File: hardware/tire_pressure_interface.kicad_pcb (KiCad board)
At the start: 2 copper layers, 98 x 40.1 mm, 82 parts, among them IC1 TPS54202HDDCR, J3 FTSH-107-01-L-D-K, J4 Conn_02x02_Counter_Clockwise, J5 Micro_SD_Card_Det1, Q1 SI2347DS-T1-GE3, T1 TP_+3V3, T10 TP_+5V, T11 TP_+5V, T3 TP_VCC, T8 TP_VCC, T9 TP_+3V3, U1 STM32G0C1KCTxN, U2 LM1117-3.3, U3 XIAO-ESP32-S3-DIP, U7 ADM3057ExRW

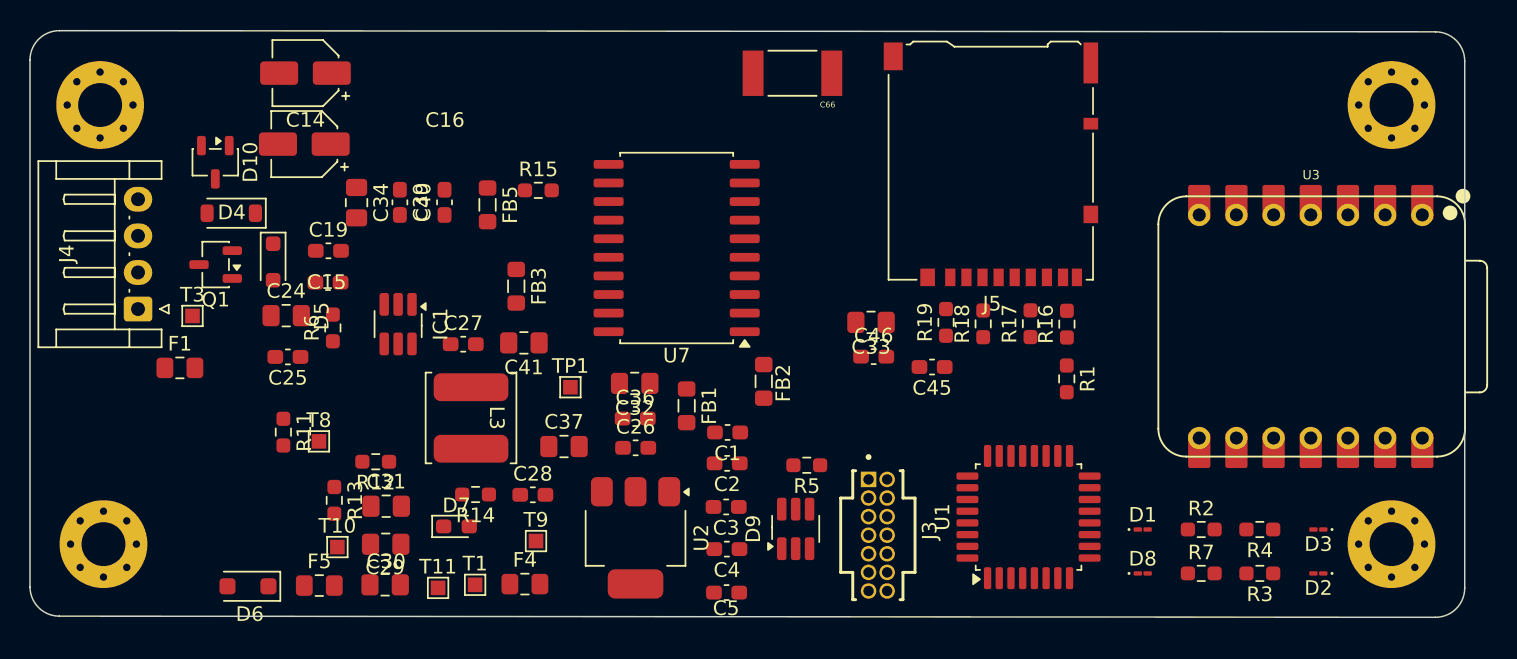
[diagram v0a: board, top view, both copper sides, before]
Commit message: pcb routing
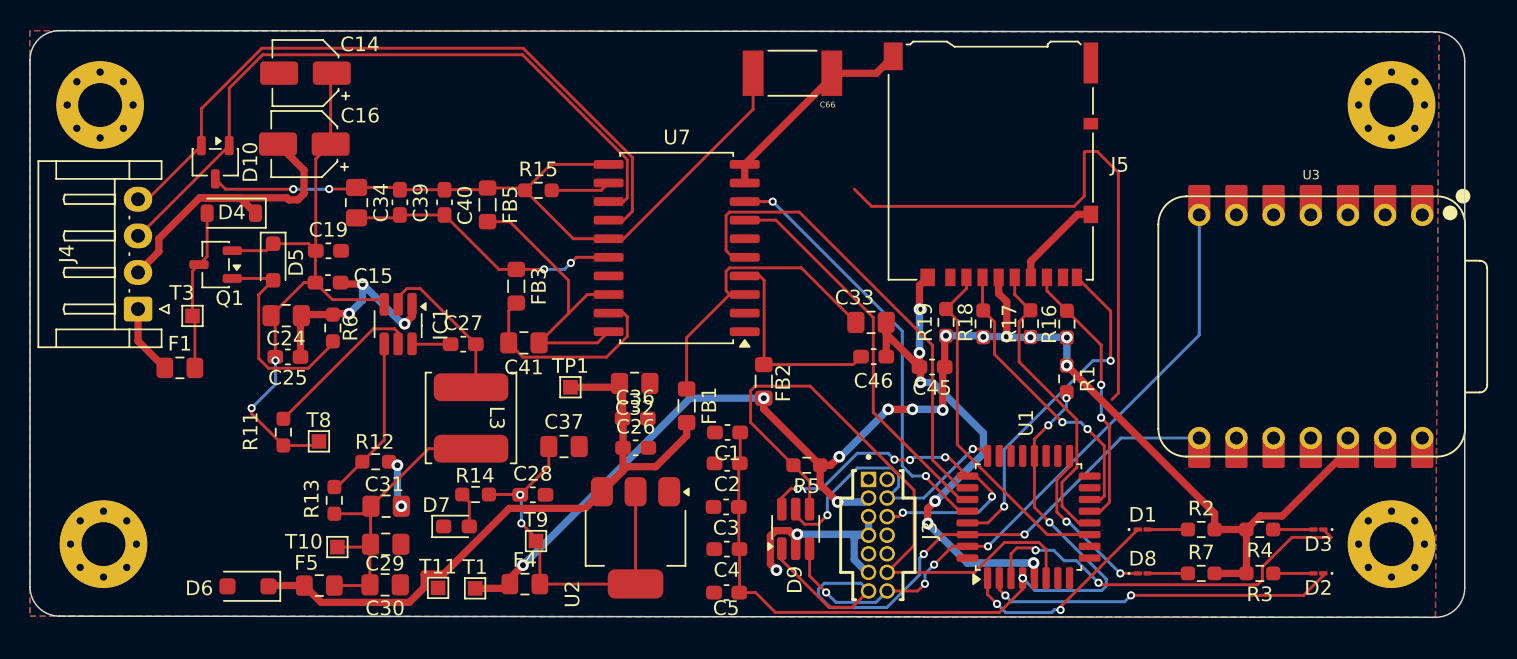
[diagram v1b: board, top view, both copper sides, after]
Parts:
- moved T1 0.24 mm to (108.4, 114.0)
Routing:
- net GND: track 0.00 -> 115.7 mm, vias 0 -> 13
- net +3V3: track 0.00 -> 98.4 mm, vias 0 -> 13
- net /STM32/STM_VCC: track 0.00 -> 54.7 mm, vias 0 -> 5
- net /CAN_BUS/GND_CAN_ISO1: track 0.00 -> 51.2 mm, vias 0 -> 2
- net /Connectors/CAN.H: track 0.00 -> 48.2 mm
- net /Connectors/CAN.L: track 0.00 -> 47.8 mm
- net +5V: track 0.00 -> 46.8 mm
- net /TX: track 0.00 -> 45.5 mm, vias 0 -> 4
- net /RX: track 0.00 -> 44.6 mm, vias 0 -> 2
- net /Connectors/RST: track 0.00 -> 44.2 mm
- net /Power/VCC_IN: track 0.00 -> 43.3 mm, vias 0 -> 2
- net (no net): track 0.00 -> 38.1 mm
- net /CAN_BUS/CAN_RX: track 0.00 -> 32.8 mm
- net /CAN_BUS/STBY_CAN_1: track 0.00 -> 29.4 mm, vias 0 -> 2
- net /STM32/LED.ERR: track 0.00 -> 27.4 mm, vias 0 -> 2
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- added copper zone on B.Cu, net GND
- added copper zone on F.Cu, net GND
